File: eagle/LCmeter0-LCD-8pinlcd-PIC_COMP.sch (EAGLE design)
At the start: 34 parts, among them IC1 PIC16F876A-X/SP-COMP-B-A/V, J1 HD44780-4BIT-8PIN, J2 PIC-UART, J3 PIC-ICSPICSP, K2 DS2Y, Q1 20MHz, T1 BC547CBE-A, X1 FREQ, X2 L/C

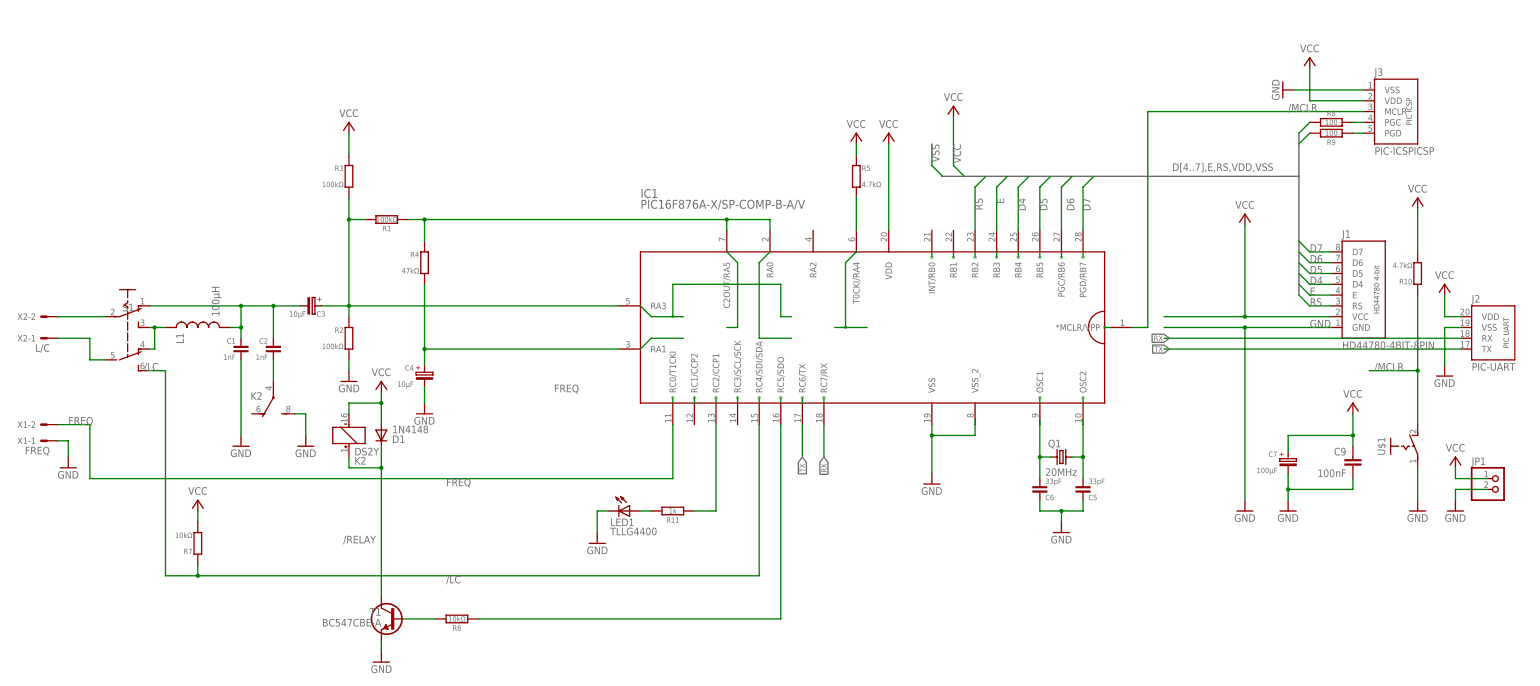
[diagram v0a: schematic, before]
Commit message: ...
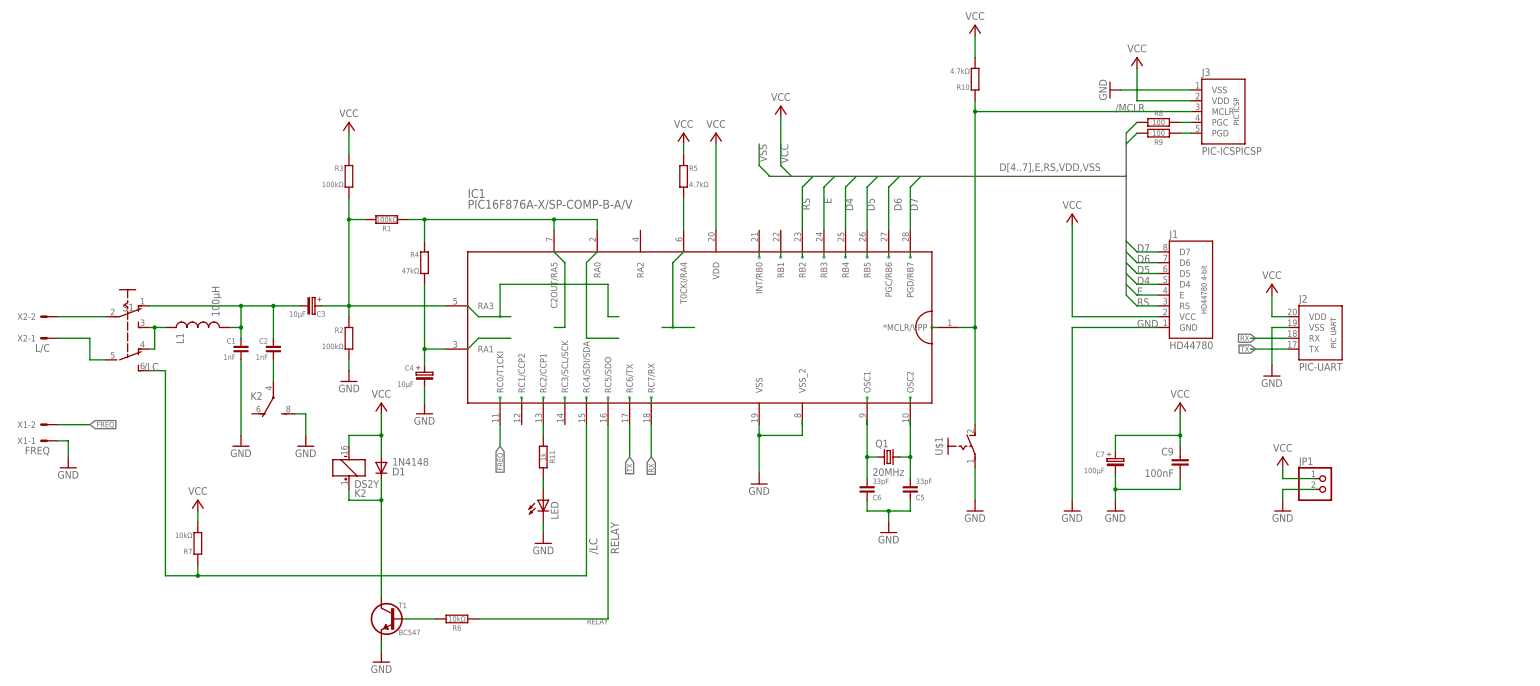
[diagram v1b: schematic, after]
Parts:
- removed LED1: TLLG4400, led:TLLG4400
- added LED: TLLG4400, led:TLLG4400
- J1: value HD44780-4BIT-8PIN -> HD44780
- T1: value BC547CBE-A -> BC547
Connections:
- net RC5 renamed RELAY
- net GND: now also LED.C; no longer LED1.C
- net N$6: now also LED.A; no longer LED1.A
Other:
- moved on the sheet: C5, C6, C7, C9, D1, IC1, J1, J2, J3, JP1, K2, Q1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
